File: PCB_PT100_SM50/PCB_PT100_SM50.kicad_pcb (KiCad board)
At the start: 2 copper layers, 80 x 65 mm, 62 parts, among them U1 TPD4E1U06DBVR, U2 INA826AIDR, U3 TPS7A4901DGNT, U4 INA826AIDR, U5 OPA2188AIDR, U6 REF3012AIDBZR, U7 TPD4E1U06DBVR, U8 78L05 5V

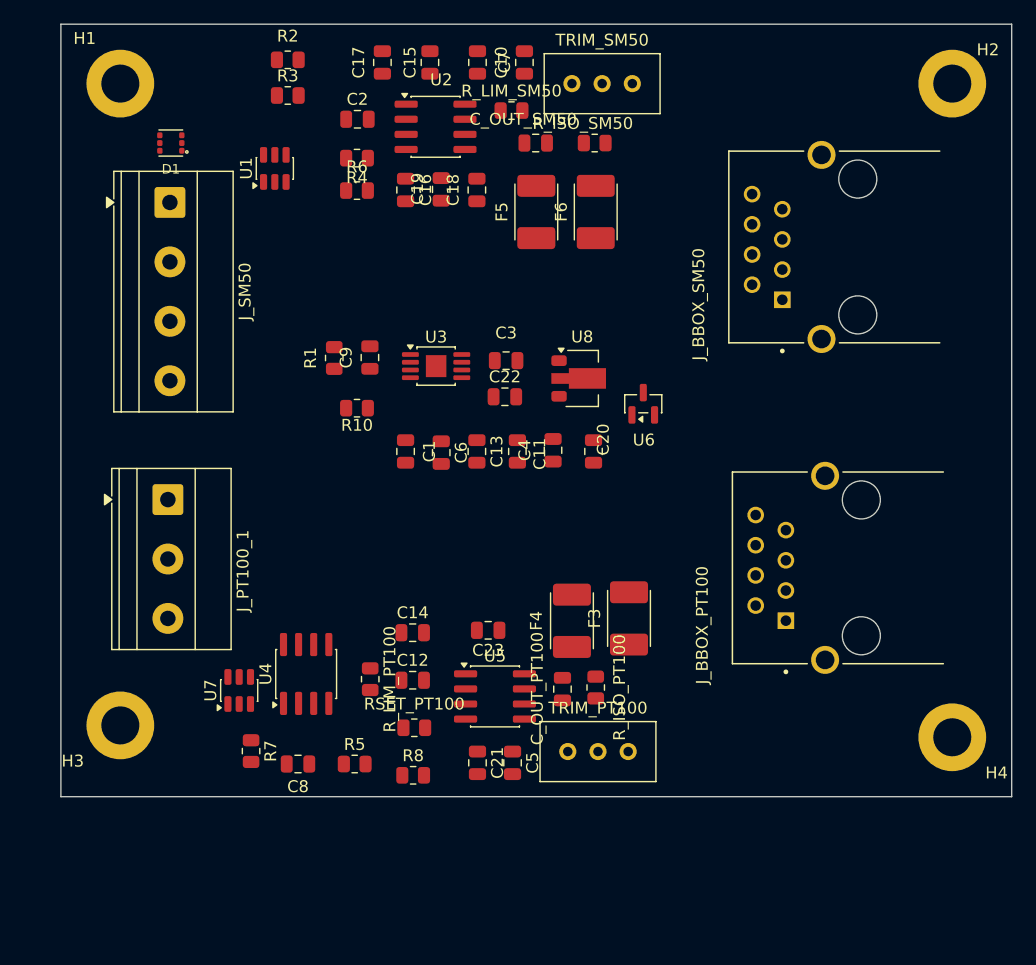
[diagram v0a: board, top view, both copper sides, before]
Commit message: Publish final PCB project
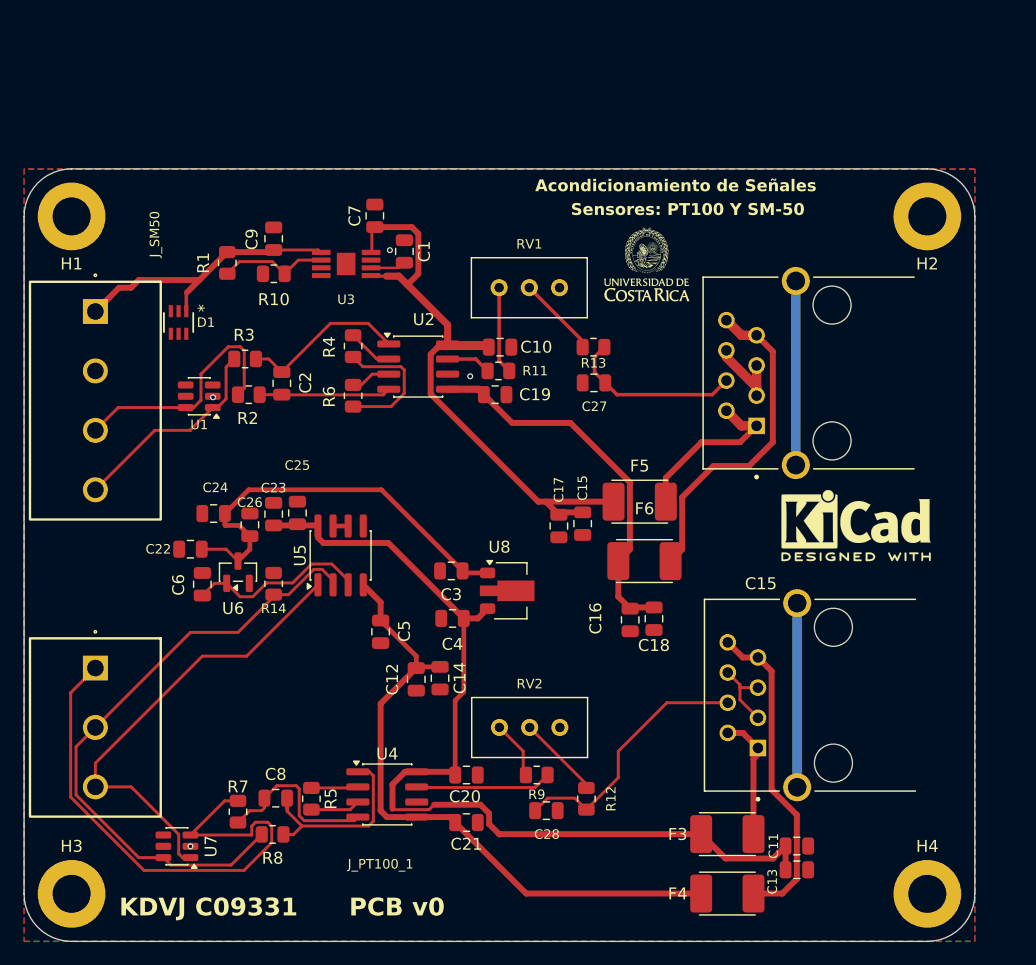
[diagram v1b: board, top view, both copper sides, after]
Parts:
- added C24: 100nF, Capacitor_SMD:C_0805_2012Metric, F.Cu at (27.9, 41.2)
- added C25: 10uF, Capacitor_SMD:C_0805_2012Metric, F.Cu at (34.9, 41.1)
- added C26: 0.1uF, Capacitor_SMD:C_0805_2012Metric, F.Cu at (30.9, 42.1)
- added G***: LOGO, Images:logoucr, F.Cu at (64.3, 20.2)
- added REF**: KiCad-Logo2_5mm_SilkScreen, Symbol:KiCad-Logo2_5mm_SilkScreen, F.Cu at (81.9, 42.2)
- J_PT100_1: footprint TerminalBlock_Phoenix:TerminalBlock_Phoenix_MKDS-1,5-3_1x03_P5.00mm_Horizontal -> ProyectoPCB:CONN_AST0250304_MZC
- J_SM50: footprint TerminalBlock_Phoenix:TerminalBlock_Phoenix_MKDS-1,5-4_1x04_P5.00mm_Horizontal -> ProyectoPCB:AST0250404
- U3: footprint Package_SO:MSOP-8-1EP_3x3mm_P0.65mm_EP1.73x1.85mm -> ProyectoPCB_Footprints:TPS7A4901DGNT_DGN8_1P89X1P57
- moved C13 44.3 mm to (76.9, 71.1), turned to 0 degrees
- moved C17 41.7 mm to (56.9, 42.2), turned to -90 degrees
- moved C15 40.9 mm to (58.9, 42.0), turned to -90 degrees
- moved C16 40.8 mm to (62.9, 50.1)
- moved C11 40.7 mm to (76.9, 69.1), turned to 0 degrees
- moved C18 39.0 mm to (64.9, 50.0)
- moved U6 36.9 mm to (29.9, 46.1)
- moved F6 29.7 mm to (64.1, 45.2), turned to 180 degrees
- moved C22 29.4 mm to (25.9, 44.2), turned to 180 degrees
- moved C20 29.2 mm to (49.1, 63.2), turned to 0 degrees
- moved R2 28.4 mm to (30.8, 31.2)
- moved F4 26.4 mm to (71.1, 73.1), turned to 180 degrees
- moved F5 25.9 mm to (63.7, 40.2), turned to 180 degrees
- moved C10 24.0 mm to (52.0, 27.2), turned to 0 degrees
- moved C2 23.1 mm to (33.6, 30.2), turned to 90 degrees
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- renumbered C_OUT_SM50 to C27, C_OUT_PT100 to C28, R_LIM_SM50 to R11, R_ISO_PT100 to R12, R_ISO_SM50 to R13, RSET_PT100 to R14, R_LIM_PT100 to R9, TRIM_SM50 to RV1, TRIM_PT100 to RV2
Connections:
- H1 pad 1: (no net) -> GND
- H2 pad 2: (no net) -> GND
- H3 pad 3: (no net) -> GND
- H4 pad 4: (no net) -> GND
- J_BBOX_PT100 pad 3: Net-(J_BBOX_PT100-GND_3) -> GND
- J_BBOX_PT100 pad 6: Net-(J_BBOX_PT100-GND_3) -> GND
- J_BBOX_SM50 pad 3: Net-(J_BBOX_SM50-GND_3) -> GND
- J_BBOX_SM50 pad 6: Net-(J_BBOX_SM50-GND_3) -> GND
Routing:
- net /+15V_PROT_PT100: track 0.00 -> 81.3 mm
- net /+15V_PROT_SM50: track 0.00 -> 55.4 mm
- net /-15V_PROT_PT100: track 0.00 -> 54.0 mm
- net /PT100_1_RETURN: track 0.00 -> 51.9 mm
- net /PT100_1_SENSE: track 0.00 -> 46.6 mm
- net /PT100_1_FORCE: track 0.00 -> 38.4 mm
- net /+5V_REF: track 0.00 -> 35.3 mm
- net /-15V_PROT_SM50: track 0.00 -> 32.1 mm
- net /-15V_BBOX_SM50: track 0.00 -> 28.0 mm
- net /-15V_BBOX_PT100: track 0.00 -> 27.2 mm
- net /+10V_SM50: track 0.00 -> 24.9 mm
- net /PT100_OUT_P: track 0.00 -> 22.1 mm
- net /SM50_SIG_P: track 0.00 -> 20.8 mm
- net /SM50_SIG_N: track 0.00 -> 18.2 mm
- net Net-(U4--IN): track 0.00 -> 17.1 mm
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- added copper zone on B.Cu, net GND
- added copper zone on F.Cu, net GND
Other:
- outline, holes or cut-outs redrawn
- board text added: "Acondicionamiento de Señales"
- board text added: "C15"
- board text added: "KDVJ C09331 PCB v0"
- board text added: "Sensores: PT100 Y SM-50"
